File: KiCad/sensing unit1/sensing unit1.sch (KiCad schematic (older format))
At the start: 25 parts, among them J1 Conn_01x03_Male, J2 Conn_01x03_Male, J3 Conn_01x02_Male, J4 Conn_01x03_Male, J5 Conn_01x02_Male, U1 LM358, U2 LM358

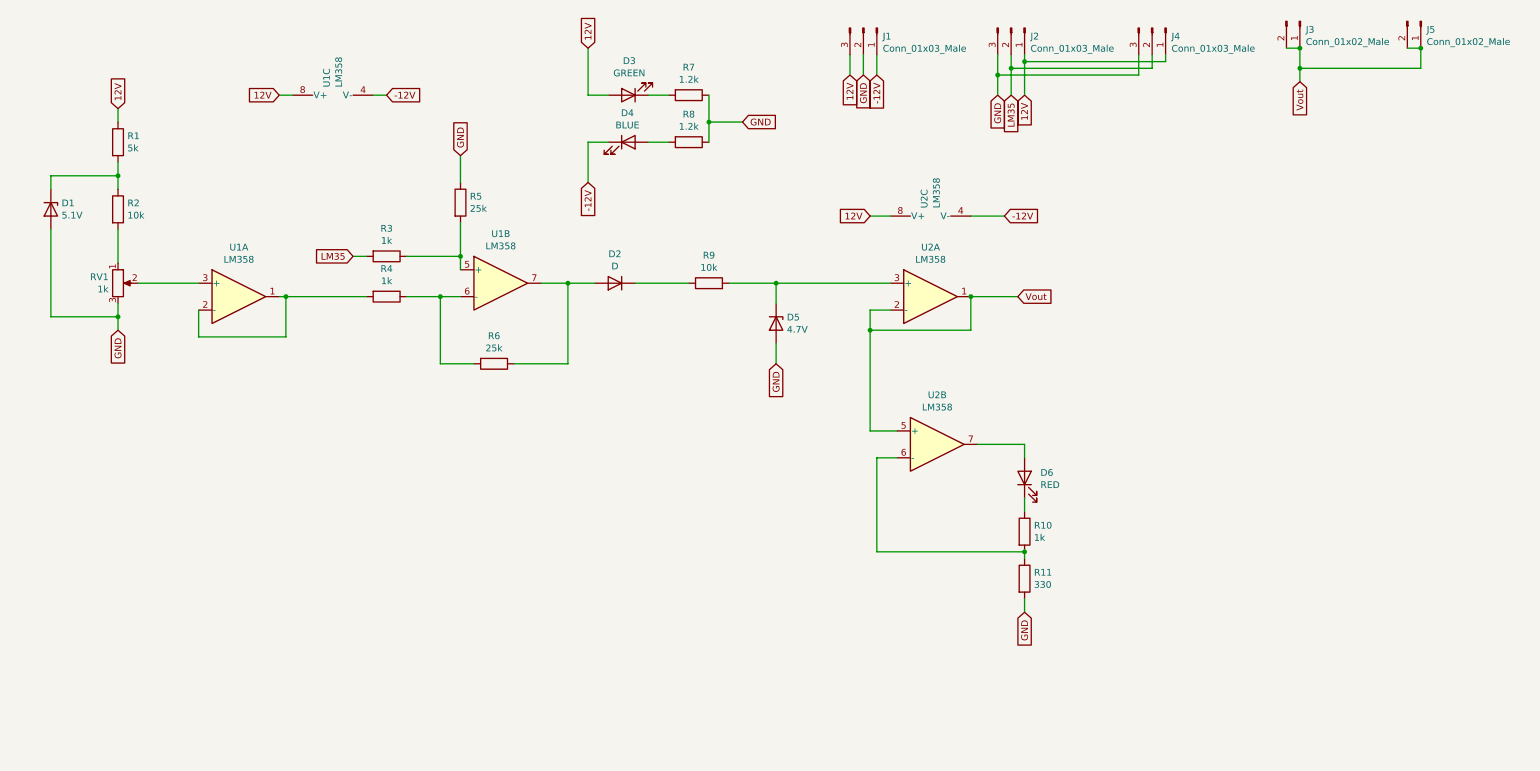
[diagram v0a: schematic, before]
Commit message: .
.
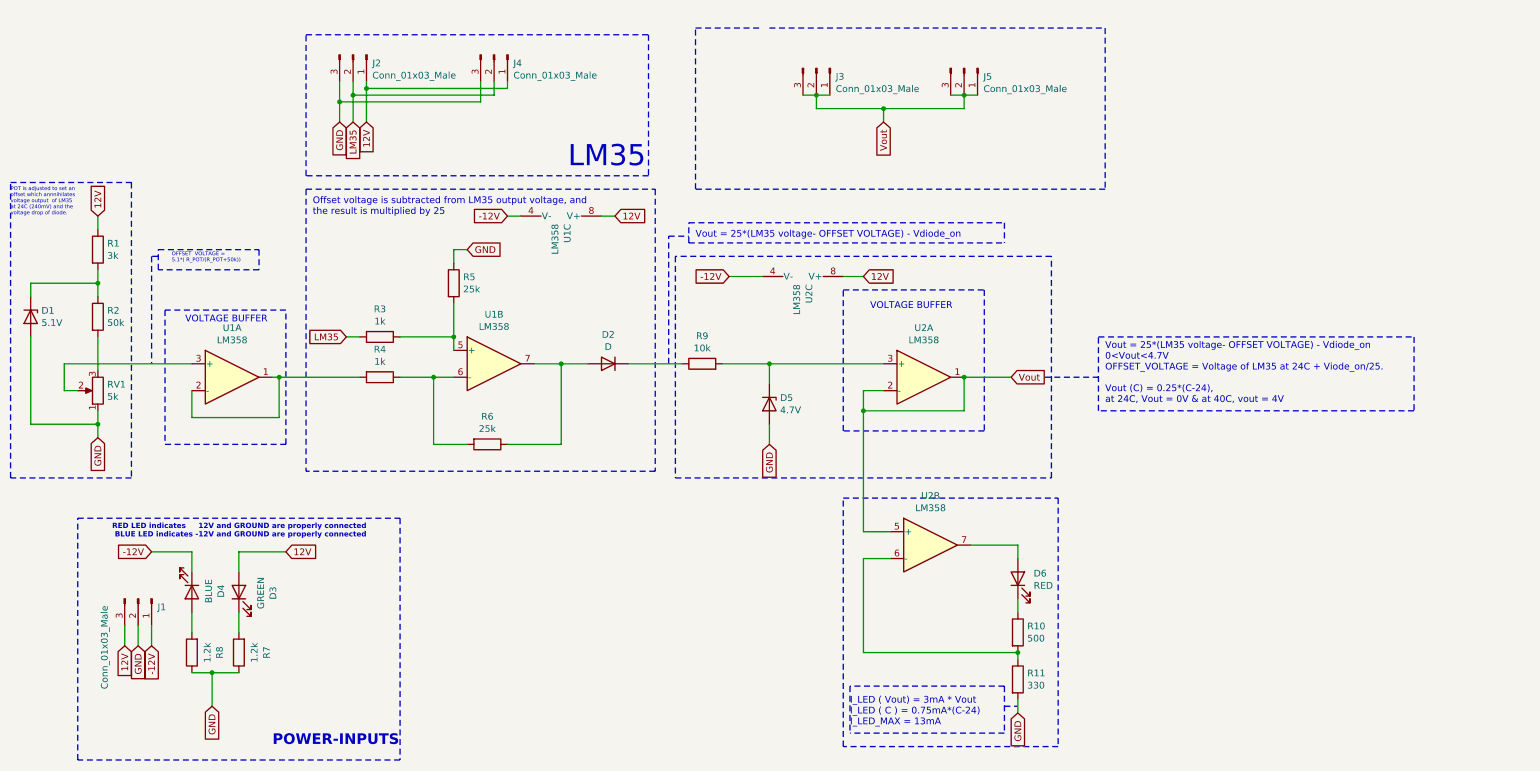
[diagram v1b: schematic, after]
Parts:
- removed J3: Conn_01x02_Male, TerminalBlock:TerminalBlock_Altech_AK300-3_P5.00mm, symbol Connector:Conn_01x02_Male
- removed J5: Conn_01x02_Male, Connector_PinHeader_2.54mm:PinHeader_1x03_P2.54mm_Vertical, symbol Connector:Conn_01x02_Male
- added J3: Conn_01x03_Male, TerminalBlock:TerminalBlock_Altech_AK300-3_P5.00mm, symbol Connector:Conn_01x03_Male
- added J5: Conn_01x03_Male, Connector_PinHeader_2.54mm:PinHeader_1x03_P2.54mm_Vertical, symbol Connector:Conn_01x03_Male
- R1: value 5k -> 3k
- R10: value 1k -> 500
- R2: value 10k -> 50k
- RV1: value 1k -> 5k; footprint Resistor_THT:R_Axial_DIN0309_L9.0mm_D3.2mm_P12.70mm_Horizontal -> Potentiometer_THT:Potentiometer_Alps_RK163_Single_Horizontal
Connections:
- net GND: now also RV1.1; no longer RV1.3
- net Vout: now also J3.1 (Pin_1), J3.2 (Pin_2), J3.3 (Pin_3), J5.1 (Pin_1), J5.2 (Pin_2), J5.3 (Pin_3)
- net at R2.2: now also RV1.3; no longer RV1.1
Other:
- note added: "I_LED ( Vout) = 3mA * Vout\nI_LED ( C ) = 0.75mA*(C-24)\nI_LED_MAX = 13mA"
- note added: "LM35"
- note added: "OFFSET VOLTAGE =\n5.1*( R_POT/(R_POT+50k))"
- note added: "Offset voltage is subtracted from LM35 output voltage, and \nthe result is multiplied by 25"
- note added: "POT is adjusted to set an \noffset which annnihilates \nvoltage output of LM35\nat 24C (240mV) and the \nvoltage drop of diode.\n"
- note added: "POWER-INPUTS"
- note added: "RED LED indicates 12V and GROUND are properly connected\nBLUE LED indicates -12V and GROUND are properly connected\n"
- note added: "VOLTAGE BUFFER"
- note added: "Vout = 25*(LM35 voltage- OFFSET VOLTAGE) - Vdiode_on\n0<Vout<4.7V\nOFFSET_VOLTAGE = Voltage of LM35 at 24C + Viode_on/25.\n\nVout (C) = 0.25*(C-24), \nat 24C, Vout = 0V & at 40C, vout = 4V"
- note added: "Vout = 25*(LM35 voltage- OFFSET VOLTAGE) - Vdiode_on\n\n"
- moved on the sheet: D1, D2, D3, D4, D5, D6, J1, J2, J4, R1, R10, R11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
